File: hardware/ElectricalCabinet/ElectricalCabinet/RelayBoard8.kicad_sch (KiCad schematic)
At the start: 0 parts

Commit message: Further wiring updates
Populated 6100 Bus
Corrected number of relay boards
Added 110v outputs to relay boards and noted light positon
Uploaded light scheme to documents folder
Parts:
- added C8: 0.1uF, Capacitor_SMD:C_0805_2012Metric, symbol Device:C
- added D57, D58, D59, D60, D61, D62, D63, D64: LED, LED_SMD:LED_0805_2012Metric, symbol Device:LED
- added J16: Screw_Terminal_01x06, TerminalBlock:TerminalBlock_MaiXu_MX126-5.0-06P_1x06_P5.00mm, symbol Connector:Screw_Terminal_01x06
- added J17: Screw_Terminal_01x09, TerminalBlock:TerminalBlock_MaiXu_MX126-5.0-09P_1x09_P5.00mm, symbol Connector:Screw_Terminal_01x09
- added K57, K58, K59, K60, K61, K62, K63, K64: G3MB-202P DC5, TrafficLightLibrary:G3MB_202P_DC5, symbol TrafficLightLibrary:G3MB-202P_DC5
- added R57, R58, R59, R60, R61, R62, R63, R64: 1kΩ, Resistor_SMD:R_0805_2012Metric, symbol Device:R
- added U9: TPIC6B595N, TrafficLightLibrary:TPIC6B595N, symbol TrafficLightLibrary:TPIC6B595N
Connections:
- new net: D60.1 (K), R60.1
- new net: D57.2 (A), D58.2 (A), D59.2 (A), D60.2 (A), D61.2 (A), D62.2 (A), D63.2 (A), D64.2 (A), K57.3, K58.3, K59.3, K60.3, K61.3, K62.3, K63.3, K64.3
- new net: D63.1 (K), R63.1
- new net: K63.4, R63.2, U9.16 (DRAIN6)
- new net: D59.1 (K), R59.1
- new net: K59.4, R59.2, U9.6 (DRAIN2)
- new net: D62.1 (K), R62.1
- new net: K62.4, R62.2, U9.15 (DRAIN5)
- new net: J17.9 (Pin_9), K57.1, K58.1, K59.1, K60.1, K61.1, K62.1, K63.1, K64.1
- new net: J17.7 (Pin_7), K63.2
- new net: D57.1 (K), R57.1
- new net: K57.4, R57.2, U9.4 (DRAIN0)
- new net: D64.1 (K), R64.1
- new net: K64.4, R64.2, U9.17 (DRAIN7)
- new net: J17.4 (Pin_4), K60.2
- new net: K60.4, R60.2, U9.7 (DRAIN3)
- new net: D58.1 (K), R58.1
- new net: J17.8 (Pin_8), K64.2
- new net: J17.1 (Pin_1), K57.2
- new net: J17.2 (Pin_2), K58.2
- new net: J17.3 (Pin_3), K59.2
- new net: J17.5 (Pin_5), K61.2
- new net: J17.6 (Pin_6), K62.2
- new net: D61.1 (K), R61.1
- new net: K61.4, R61.2, U9.14 (DRAIN4)
- new net: C8.1, J16.2 (Pin_2), U9.10 (GND), U9.11 (GND), U9.19 (GND), U9.9 (~{G})
- new net: J16.4 (Pin_4), U9.12 (RCK)
- new net: J16.3 (Pin_3), U9.13 (SRCK)
- new net: J16.1 (Pin_1), U9.18 (SEROUT)
- new net: C8.2, J16.6 (Pin_6), U9.2 (VCC), U9.8 (~{SRCLR})
- new net: K58.4, R58.2, U9.5 (DRAIN1)
- new net SERIN: J16.5 (Pin_5), U9.3 (SERIN)
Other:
- note added: "RELAY MODULE 8"

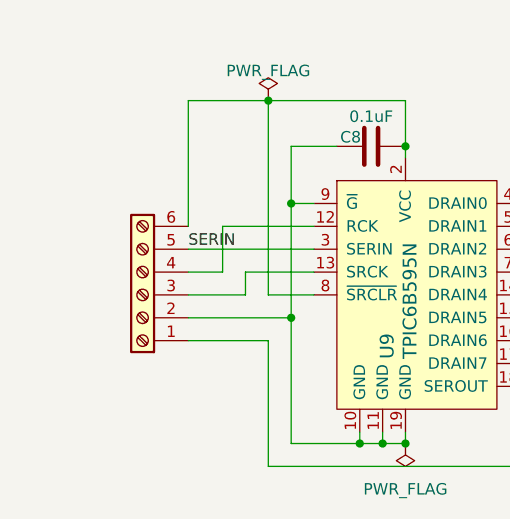
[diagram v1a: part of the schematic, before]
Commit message: Electrical Cabinet done
Electrical Cabinet done, let me know if there are any changes or mistakes.
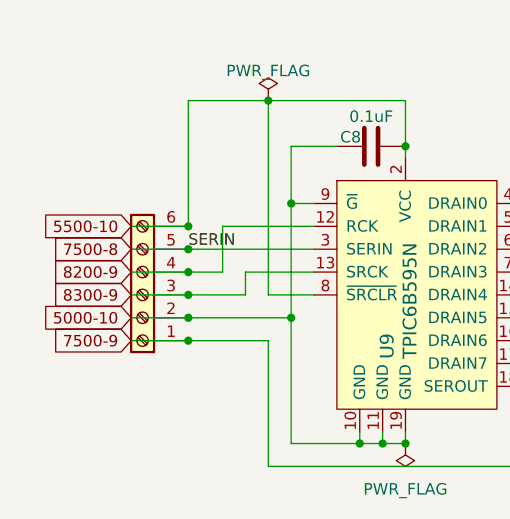
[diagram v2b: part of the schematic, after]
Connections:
- net 5000-10: now reaches C8.1, J16.2 (Pin_2), U9.10 (GND), U9.11 (GND), U9.19 (GND), U9.9 (~{G})
- net 8200-9: now reaches J16.4 (Pin_4), U9.12 (RCK)
- net 8300-9: now reaches J16.3 (Pin_3), U9.13 (SRCK)
- net 7500-9: now reaches J16.1 (Pin_1), U9.18 (SEROUT)
- net 5500-10: now reaches C8.2, J16.6 (Pin_6), U9.2 (VCC), U9.8 (~{SRCLR})
- net SERIN renamed 7500-8
